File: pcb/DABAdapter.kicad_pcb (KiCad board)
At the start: 2 copper layers, 27 x 58.5 mm, 33 parts, among them J1 RFShield_OnePiece, J2 Ant, J3 Conn_01x06, J4 AudioJack3_Ground, J5 TRS Antenna, J6 Conn_01x06, U1 SST25VF080B-50-4x-S2Ax, U3 abcdefg, U4 MIC5504-1.8YM5, Y1 19.2Mhz

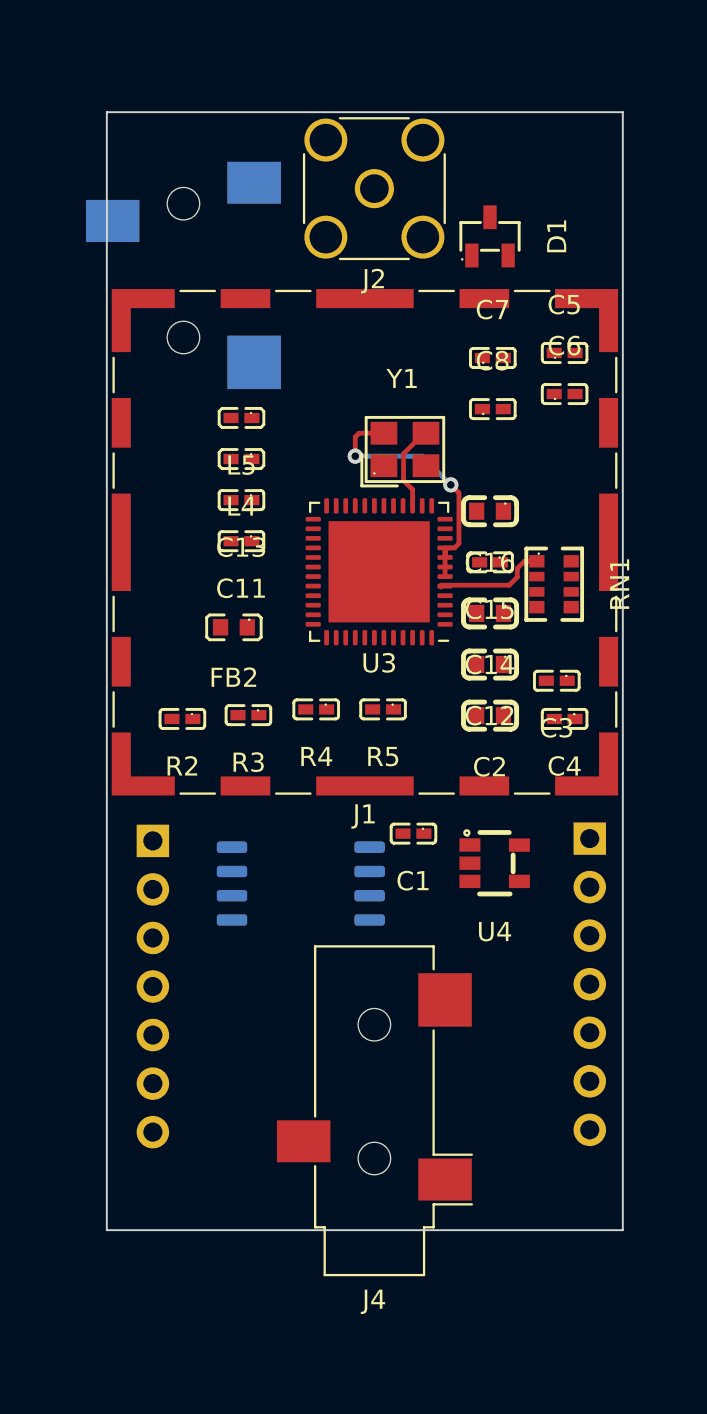
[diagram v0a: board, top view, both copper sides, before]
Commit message: Routing of the pcb
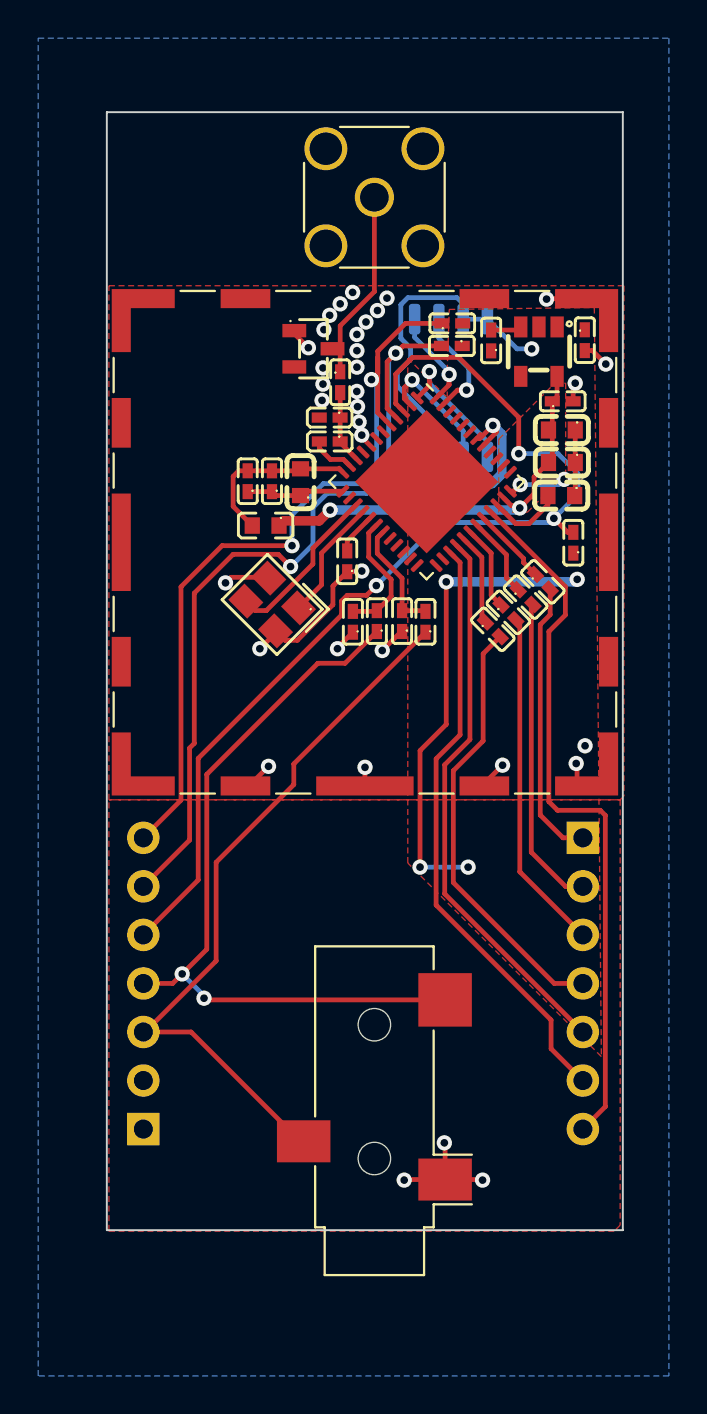
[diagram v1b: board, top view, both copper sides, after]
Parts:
- removed J5: TRS Antenna, Connector_Audio:Jack_3.5mm_CUI_SJ-3523-SMT_Horizontal
- removed RN1: 10k, jlc_footprints:RES-ARRAY-SMD_0603-8P-L3.2-W1.6-BL
- added R1: 10k, jlc_footprints:C0402, F.Cu at (117.7, 73.8)
- added R6: 10k, jlc_footprints:C0402, F.Cu at (122.0, 84.4)
- added R7: 10k, jlc_footprints:C0402, F.Cu at (115.6, 74.1)
- added R8: 10k, jlc_footprints:C0402, F.Cu at (115.7, 72.9)
- moved U1 27.1 mm to (115.6, 76.3), turned to 90 degrees
- moved U4 26.9 mm to (120.2, 74.4), turned to 90 degrees
- moved R2 17.9 mm to (118.6, 88.0), turned to -45 degrees
- moved C3 17.9 mm to (122.6, 73.8), turned to -90 degrees
- moved C5 17.1 mm to (111.7, 88.5), turned to 90 degrees
- moved C4 16.6 mm to (121.4, 77.0), turned to 0 degrees
- moved R3 15.8 mm to (119.5, 87.2), turned to -45 degrees
- moved J3 15.1 mm to (99.5, 115.1), turned to 0 degrees
- moved C1 14.7 mm to (110.2, 85.4), turned to 90 degrees
- moved C7 14.6 mm to (113.0, 88.5), turned to 90 degrees
- moved C6 14.0 mm to (114.3, 88.5), turned to 90 degrees
- moved R4 13.6 mm to (120.4, 86.4), turned to -45 degrees
- moved C8 13.3 mm to (110.5, 88.5), turned to 90 degrees
- moved C15 12.2 mm to (106.2, 81.2), turned to 90 degrees
- moved C2 12.1 mm to (121.4, 81.9)
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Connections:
- J3 pad 3: SMODE -> ROUT
- J3 pad 4: INTB -> LOUT
- J3 pad 5: RSTB -> INTB
- J3 pad 6: LOUT -> RSTB
- J3 pad 7: ROUT -> SMODE
- J6 pad 3: SPI_SSB -> SPI_SCLK
- J6 pad 4: SPI_SCLK -> SPI_SSB
- J6 pad 5: I2S_DCLK -> I2S_DFS
- J6 pad 6: I2S_DFS -> I2S_DCLK
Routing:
- net INTB: track 0.10 -> 54.5 mm, vias 0 -> 3
- net +3V3: track 0.00 -> 46.9 mm, vias 0 -> 6
- net RSTB: track 0.00 -> 43.6 mm, vias 0 -> 2
- net LOUT: track 0.00 -> 39.6 mm, vias 0 -> 2
- net ROUT: track 0.00 -> 37.8 mm
- net I2S_DATA: track 0.00 -> 37.3 mm
- net SMODE: track 5.89 -> 41.7 mm, vias 0 -> 2
- net I2S_DCLK: track 0.00 -> 31.6 mm
- net I2S_DFS: track 0.00 -> 29.3 mm
- net GND: track 14.1 -> 40.3 mm, vias 2 -> 34
- net SPI_SSB: track 0.00 -> 22.8 mm
- net +1V8: track 0.00 -> 21.7 mm, vias 0 -> 2
- net SPI_SCLK: track 0.00 -> 17.9 mm
- net SPI_MOSI: track 0.00 -> 16.4 mm
- net SPI_MISO: track 0.00 -> 14.8 mm
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- added copper zone on F.Cu, net +1V8
- added copper zone on F.Cu, net +3V3
- added copper zone on B.Cu, net GND
- added copper zone on F.Cu, net GND
